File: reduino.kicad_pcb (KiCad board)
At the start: 2 copper layers, 68.6 x 53.3 mm, 35 parts, among them P1 Power, P2 Analog, P3 Digital, P4 Digital, P5 CONN_1, P6 CONN_1, P7 CONN_1, P8 CONN_1, SW1 SW_RESET, U1 ATmega32U4-AU, U2 NCP1117ST33T3G, Y1 16MHz

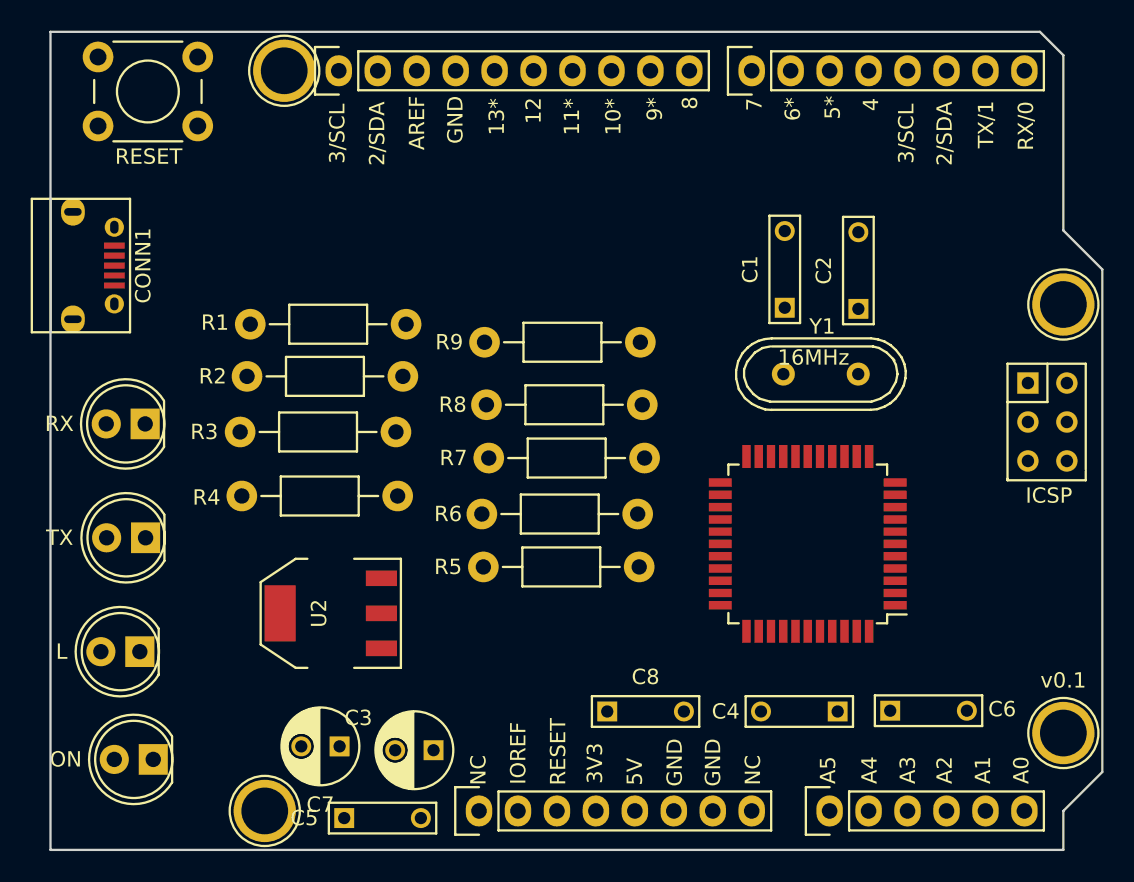
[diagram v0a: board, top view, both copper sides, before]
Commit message: Beta version
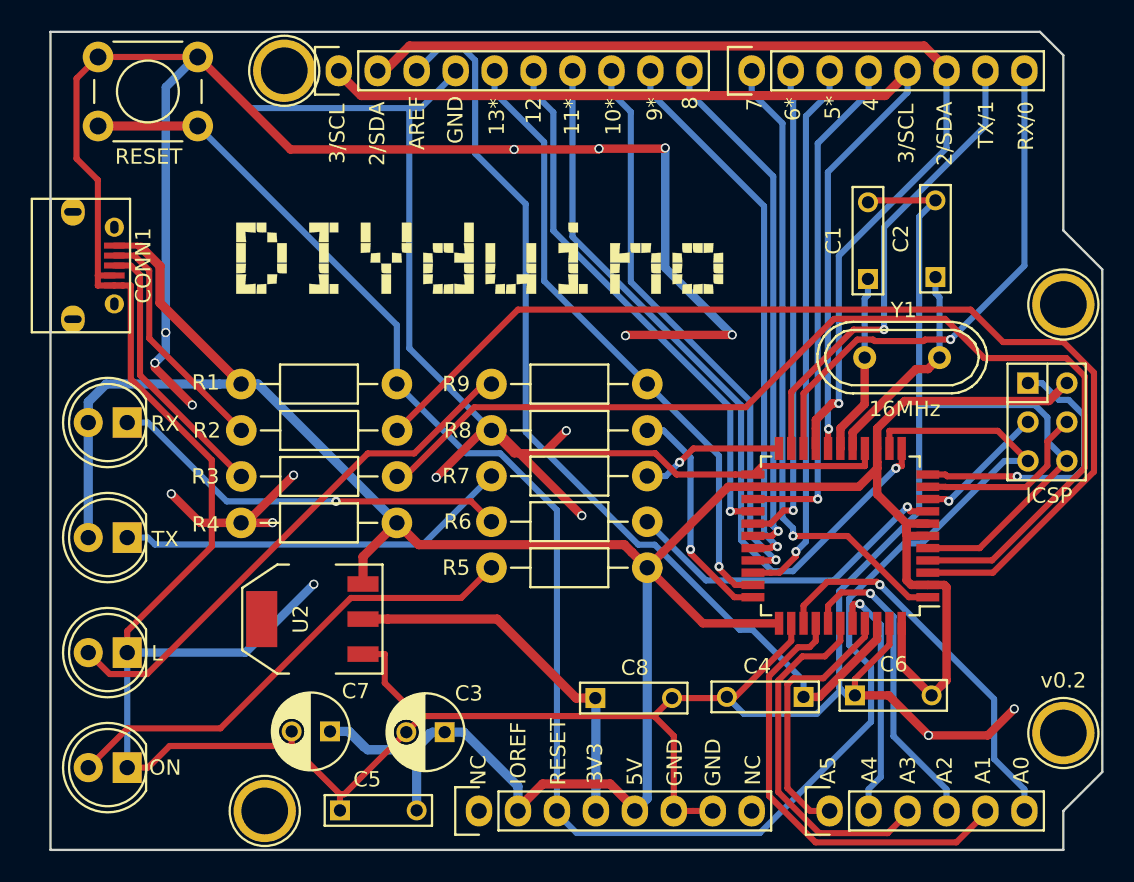
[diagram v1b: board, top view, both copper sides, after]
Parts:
- added G***: LOGO, reduino:diyduino, F.Cu at (151.3, 87.6)
- moved C1 5.74 mm to (164.3, 89.1)
- moved C2 5.44 mm to (168.7, 89.0)
- moved Y1 5.41 mm to (166.5, 94.3)
- moved R1 3.95 mm to (123.4, 96.0)
- moved R2 3.54 mm to (133.6, 99.0)
- moved R3 2.90 mm to (133.6, 102.0)
- moved R9 2.76 mm to (139.7, 96.0)
- moved C6 2.51 mm to (163.4, 116.3)
- moved C4 2.42 mm to (160.1, 116.4)
- moved U1 2.19 mm to (162.5, 105.9)
- moved D4 1.78 mm to (116.0, 121.0)
- moved R4 1.75 mm to (123.4, 105.0)
- moved R8 1.71 mm to (139.7, 99.0)
- moved C3 1.38 mm to (136.7, 118.7)
- moved U2 1.26 mm to (128.1, 111.3)
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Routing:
- net GND: track 0.00 -> 413.4 mm, vias 0 -> 17
- net +5C: track 0.00 -> 200.6 mm
- net /RESET: track 0.00 -> 121.3 mm
- net /D-: track 0.00 -> 70.4 mm
- net /D+: track 0.00 -> 69.3 mm
- net /D2: track 0.00 -> 66.9 mm, vias 0 -> 1
- net /D3: track 0.00 -> 65.4 mm, vias 0 -> 1
- net /AREF: track 0.00 -> 63.6 mm
- net /IO11: track 0.00 -> 50.5 mm, vias 0 -> 1
- net /D7: track 0.00 -> 41.9 mm, vias 0 -> 1
- net /IO13: track 0.00 -> 41.2 mm, vias 0 -> 1
- net /IO10: track 0.00 -> 37.9 mm, vias 0 -> 1
- net /IO9: track 0.00 -> 36.1 mm, vias 0 -> 1
- net /D5: track 0.00 -> 35.8 mm, vias 0 -> 1
- net /IO12: track 0.00 -> 35.5 mm, vias 0 -> 1
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- added copper zone on B.Cu, net GND
- added copper zone on F.Cu, net GND
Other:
- net class Default: trace_width 0.4 -> 0.55
- board text added: "v0.2"
- board text removed: "v0.1"
